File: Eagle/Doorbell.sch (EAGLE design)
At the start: 33 parts

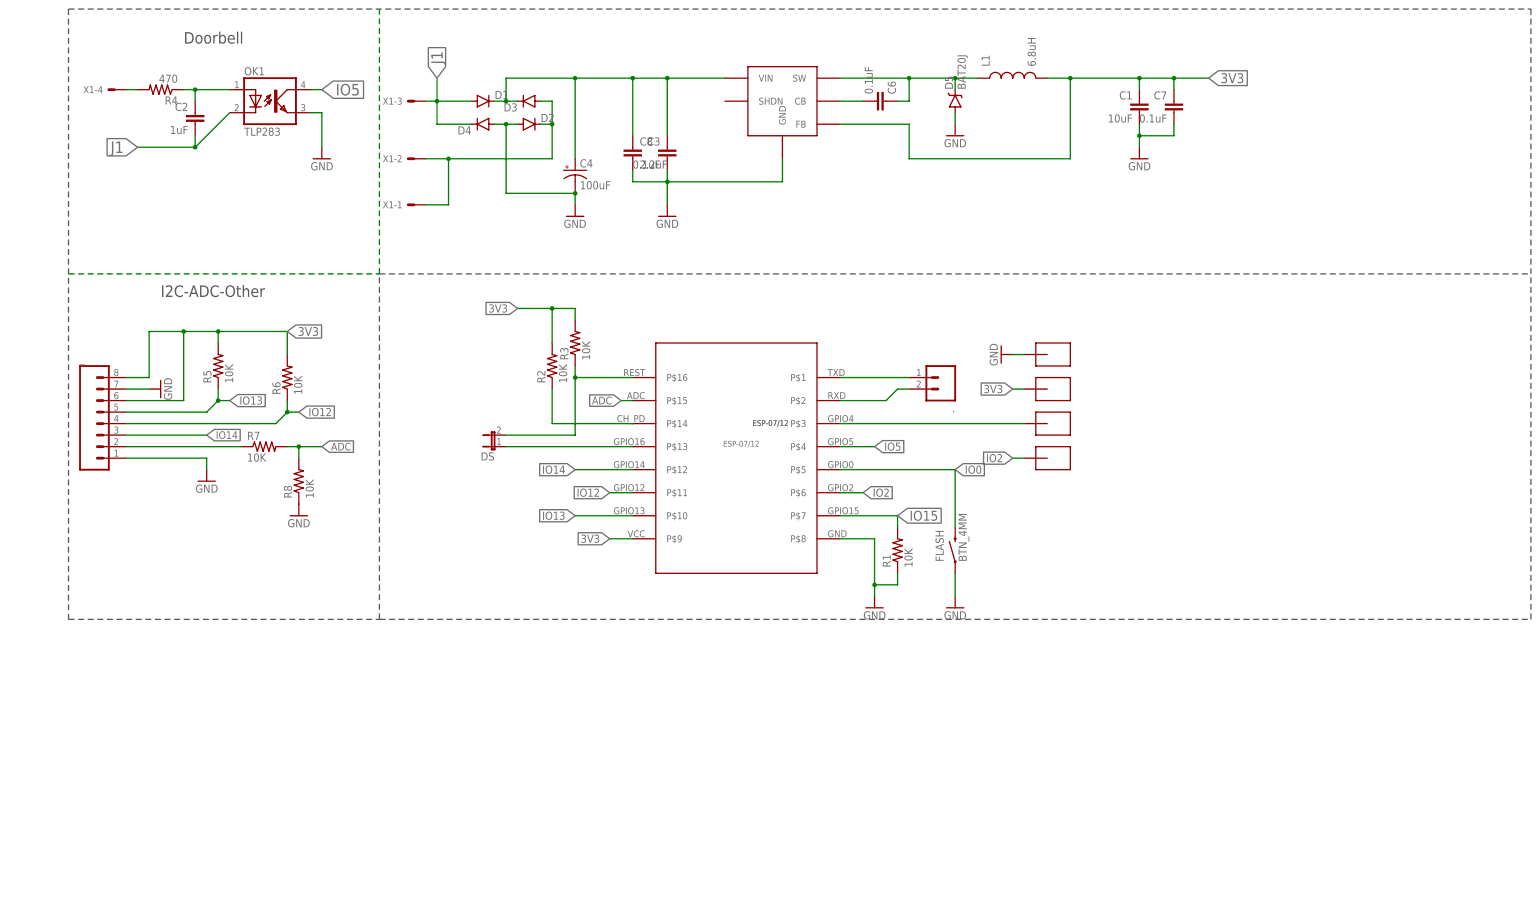
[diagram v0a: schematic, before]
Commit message: Add files via upload
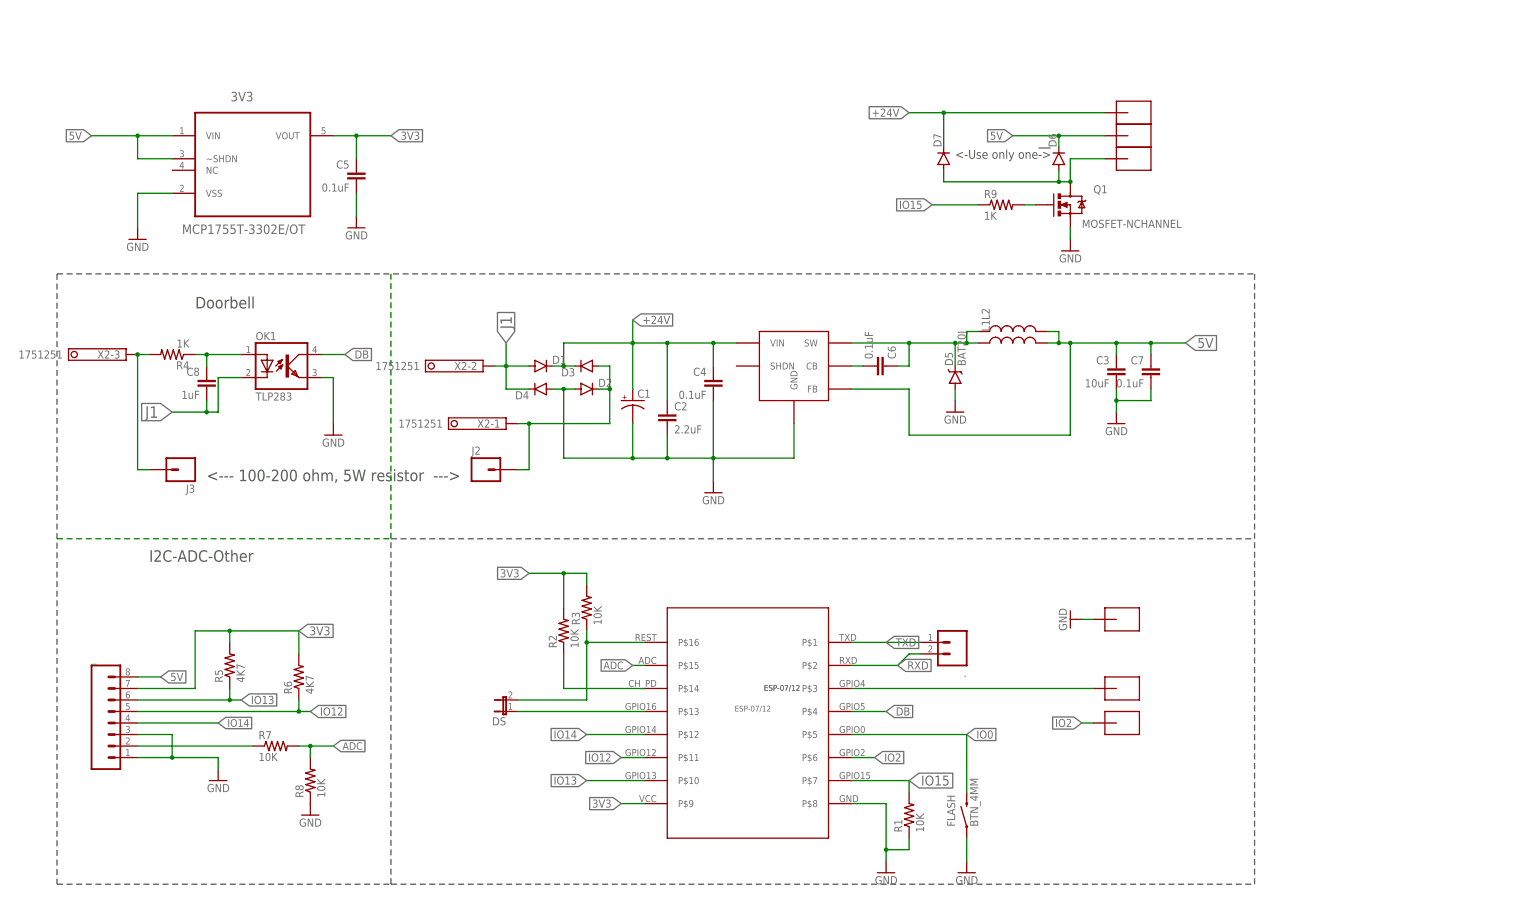
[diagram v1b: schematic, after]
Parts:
- removed X1: (no value), con-molex:KK-156-4
- added 3V3: MCP1755T-3302E/OT, Microchip_By_element14_Batch_1:MCP1801T-3302I/OT
- added C5: 0.1uF, SparkFun-Capacitors:CAP
- added D6, D7: (no value), SparkFun-DiscreteSemi:DIODESOD123
- added J2, J3: (no value), SparkFun-Connectors:M01SMDNS
- added L2: (no value), SparkFun-Passives:INDUCTOR0805
- added Q1: MOSFET-NCHANNEL, SparkFun-DiscreteSemi:MOSFET-NCHANNELAO3404A
- added R9: 1K, SparkFun-Resistors:RESISTOR0805-RES
- added U$6, U$7: SMD-PAD-SM, CuriousTech:SMD-PAD-SM
- added X2: 1751251, con-phoenix-350:1751251
- C1: value 10uF -> (none); device SparkFun-Capacitors:CAP -> SparkFun-Capacitors:CAP_POLPTH4
- C2: value 1uF -> 2.2uF; device SparkFun-Capacitors:CAP -> SparkFun-Passives:CAP1206
- C3: value 0.1uF -> 10uF
- C4: value 100uF -> 0.1uF; device SparkFun-Passives:CAP_POLF80 -> SparkFun-Capacitors:CAP
- C8: value 2.2uF -> 1uF; device SparkFun-Passives:CAP1206 -> SparkFun-Capacitors:CAP
- L1: value 6.8uH -> (none); device SparkFun-Passives:INDUCTOR1007 -> SparkFun-Passives:INDUCTOR0805
- R4: value 470 -> 1K
- R5, R6: value 10K -> 4K7
- VREG: value LMR16006YQ3DDCRQ1 -> LMR16006YQ5DDCRQ1
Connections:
- net IO5 renamed DB
- new net 5V: 3V3.VIN, 3V3.~SHDN, C3.1, C7.1, D6.C, L1.2, L2.2, U$7.P$1, VREG.FB, _.8
- new net N$1: D6.A, D7.A, Q1.D, U$6.P$1
- new net N$8: Q1.G, R9.2
- net +24V: now also C1.+, C2.1, C4.1, D7.C, U$3.P$1; no longer C3.1, C4.+, C8.1
- net 3V3: now also 3V3.VOUT, C5.1, _.7; no longer C1.1, C7.1, L1.2, U$3.P$1, VREG.FB, _.6, _.8
- net GND: now also 3V3.VSS, C1.-, C2.2, C4.2, C5.2, Q1.S, _.3; no longer C1.2, C4.-, C8.2, _.7
- net IO12: now also _.5; no longer _.4
- net IO13: now also _.6; no longer _.5
- net IO14: now also _.4; no longer _.3
- net IO15: now also R9.1
- net J1: now also C8.2, X2-2.K; no longer C2.2, X1-3.S
- net N$2: now also C8.1; no longer C2.1
- net N$3: now also J2.1, X2-1.K; no longer X1-1.S, X1-2.S
- net N$5: now also J3.1, X2-3.K; no longer X1-4.S
- net N$7: now also L2.1
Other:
- note added: "<--- 100-200 ohm, 5W resistor --->"
- note added: "<-Use only one!->"
- moved on the sheet: ., C2, C3, C6, C7, C8, D1, D2, D3, D4, D5, DS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
